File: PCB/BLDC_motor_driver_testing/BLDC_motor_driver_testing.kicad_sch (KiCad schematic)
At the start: 18 parts, among them J1 PWR, J2 PHASE A, J3 PHASE B, J4 PHASE C, U1 AMS1117-3.3

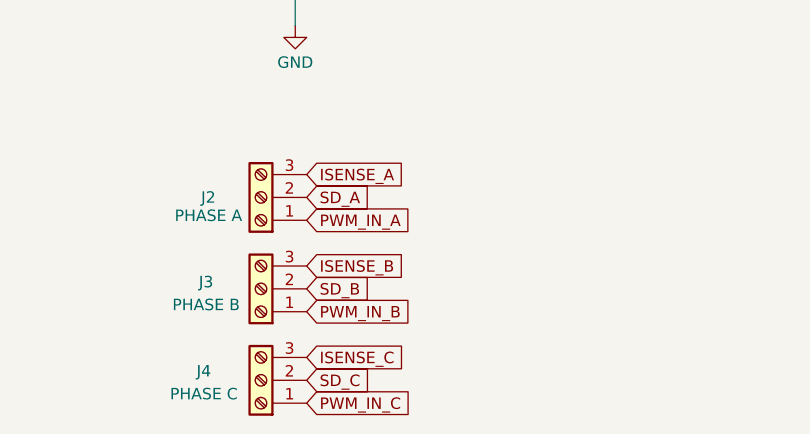
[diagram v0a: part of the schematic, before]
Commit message: Getting closer to finish 2 ;)
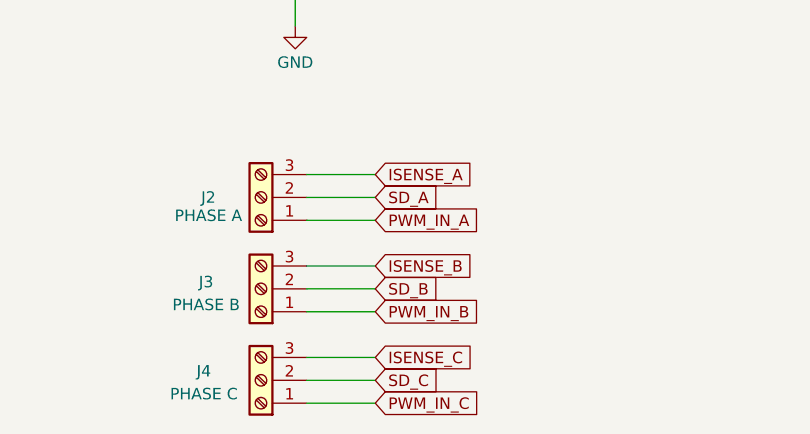
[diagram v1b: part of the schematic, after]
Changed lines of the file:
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@@
+	(wire
+		(pts
+			(xy 125.73 147.32) (xy 118.11 147.32)
+		)
+		(stroke
+			(width 0)
+			(type default)
+		)
+	)
 	(wire
 		(pts
@@
 	(wire
 		(pts
+			(xy 125.73 144.78) (xy 118.11 144.78)
+		)
+		(stroke
+			(width 0)
+			(type default)
+		)
+	)
+	(wire
+		(pts
 			(xy 194.31 78.74) (xy 194.31 83.82)
 		)
@@
 	(wire
 		(pts
+			(xy 125.73 124.46) (xy 118.11 124.46)
+		)
+		(stroke
+			(width 0)
+			(type default)
+		)
+	)
+	(wire
+		(pts
 			(xy 186.69 90.17) (xy 186.69 87.63)
 		)
@@
 	(wire
 		(pts
+			(xy 125.73 127) (xy 118.11 127)
+		)
+		(stroke
+			(width 0)
+			(type default)
+		)
+	)
+	(wire
+		(pts
 			(xy 156.21 101.6) (xy 142.24 101.6)
 		)
@@
 	(wire
 		(pts
+			(xy 125.73 137.16) (xy 118.11 137.16)
+		)
+		(stroke
+			(width 0)
+			(type default)
+		)
+	)
+	(wire
+		(pts
 			(xy 73.66 96.52) (xy 76.2 96.52)
 		)
@@
 	(wire
 		(pts
+			(xy 125.73 132.08) (xy 118.11 132.08)
+		)
+		(stroke
+			(width 0)
+			(type default)
+		)
+	)
+	(wire
+		(pts
 			(xy 129.54 48.26) (xy 135.89 48.26)
 		)
@@
 	(wire
 		(pts
+			(xy 125.73 134.62) (xy 118.11 134.62)
+		)
+		(stroke
+			(width 0)
+			(type default)
+		)
+	)
+	(wire
+		(pts
 			(xy 207.01 132.08) (xy 212.09 132.08)
 		)
@@
 		(pts
 			(xy 76.2 90.17) (xy 76.2 93.98)
+		)
+		(stroke
+			(width 0)
+			(type default)
+		)
+	)
+	(wire
+		(pts
+			(xy 125.73 121.92) (xy 118.11 121.92)
+		)
+		(stroke
+			(width 0)
+			(type default)
+		)
+	)
+	(wire
+		(pts
+			(xy 125.73 142.24) (xy 118.11 142.24)
 		)
 		(stroke
@@
 	(global_label "SD_B"
 		(shape input)
-		(at 118.11 134.62 0)
+		(at 125.73 134.62 0)
 		(fields_autoplaced yes)
 		(effects
@@
 		)
 		(property "Intersheetrefs" "${INTERSHEET_REFS}"
-			(at 125.8123 134.62 0)
+			(at 133.4323 134.62 0)
 			(effects
 				(font
@@
 	(global_label "SD_A"
 		(shape input)
-		(at 118.11 124.46 0)
+		(at 125.73 124.46 0)
 		(fields_autoplaced yes)
 		(effects
@@
 		)
 		(property "Intersheetrefs" "${INTERSHEET_REFS}"
-			(at 125.6309 124.46 0)
+			(at 133.2509 124.46 0)
 			(effects
 				(font
@@
 	(global_label "PWM_IN_B"
 		(shape input)
-		(at 118.11 137.16 0)
+		(at 125.73 137.16 0)
 		(fields_autoplaced yes)
 		(effects
@@
 		)
 		(property "Intersheetrefs" "${INTERSHEET_REFS}"
-			(at 130.4085 137.16 0)
+			(at 138.0285 137.16 0)
 			(effects
 				(font
@@
 	(global_label "ISENSE_B"
 		(shape input)
-		(at 118.11 132.08 0)
+		(at 125.73 132.08 0)
 		(fields_autoplaced yes)
 		(effects
@@
 		)
 		(property "Intersheetrefs" "${INTERSHEET_REFS}"
-			(at 129.9851 132.08 0)
+			(at 137.6051 132.08 0)
 			(effects
 				(font
@@
 	(global_label "PWM_IN_A"
 		(shape input)
-		(at 118.11 127 0)
+		(at 125.73 127 0)
 		(fields_autoplaced yes)
 		(effects
@@
 		)
 		(property "Intersheetrefs" "${INTERSHEET_REFS}"
-			(at 130.2271 127 0)
+			(at 137.8471 127 0)
 			(effects
 				(font
@@
 	(global_label "ISENSE_A"
 		(shape input)
-		(at 118.11 121.92 0)
+		(at 125.73 121.92 0)
 		(fields_autoplaced yes)
 		(effects
@@
 		)
 		(property "Intersheetrefs" "${INTERSHEET_REFS}"
-			(at 129.8037 121.92 0)
+			(at 137.4237 121.92 0)
 			(effects
 				(font
@@
 	(global_label "ISENSE_C"
 		(shape input)
-		(at 118.11 142.24 0)
+		(at 125.73 142.24 0)
 		(fields_autoplaced yes)
 		(effects
@@
 		)
 		(property "Intersheetrefs" "${INTERSHEET_REFS}"
-			(at 129.9851 142.24 0)
+			(at 137.6051 142.24 0)
 			(effects
 				(font
@@
 	(global_label "PWM_IN_C"
 		(shape input)
-		(at 118.11 147.32 0)
+		(at 125.73 147.32 0)
 		(fields_autoplaced yes)
 		(effects
@@
 		)
 		(property "Intersheetrefs" "${INTERSHEET_REFS}"
-			(at 130.4085 147.32 0)
+			(at 138.0285 147.32 0)
 			(effects
 				(font
@@
 	(global_label "SD_C"
 		(shape input)
-		(at 118.11 144.78 0)
+		(at 125.73 144.78 0)
 		(fields_autoplaced yes)
 		(effects
@@
 		)
 		(property "Intersheetrefs" "${INTERSHEET_REFS}"
-			(at 125.8123 144.78 0)
-			(effects
-				(font
+			(at 133.4323 144.78 0)
+			(effects
+				(font
